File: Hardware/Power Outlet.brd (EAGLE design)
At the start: 160 x 100 mm, 36 parts, among them IC1 ATMega 328p-pu, IC2 ULN2003AD, K1 G5LE, K2 G5LE, Q1 16MHz

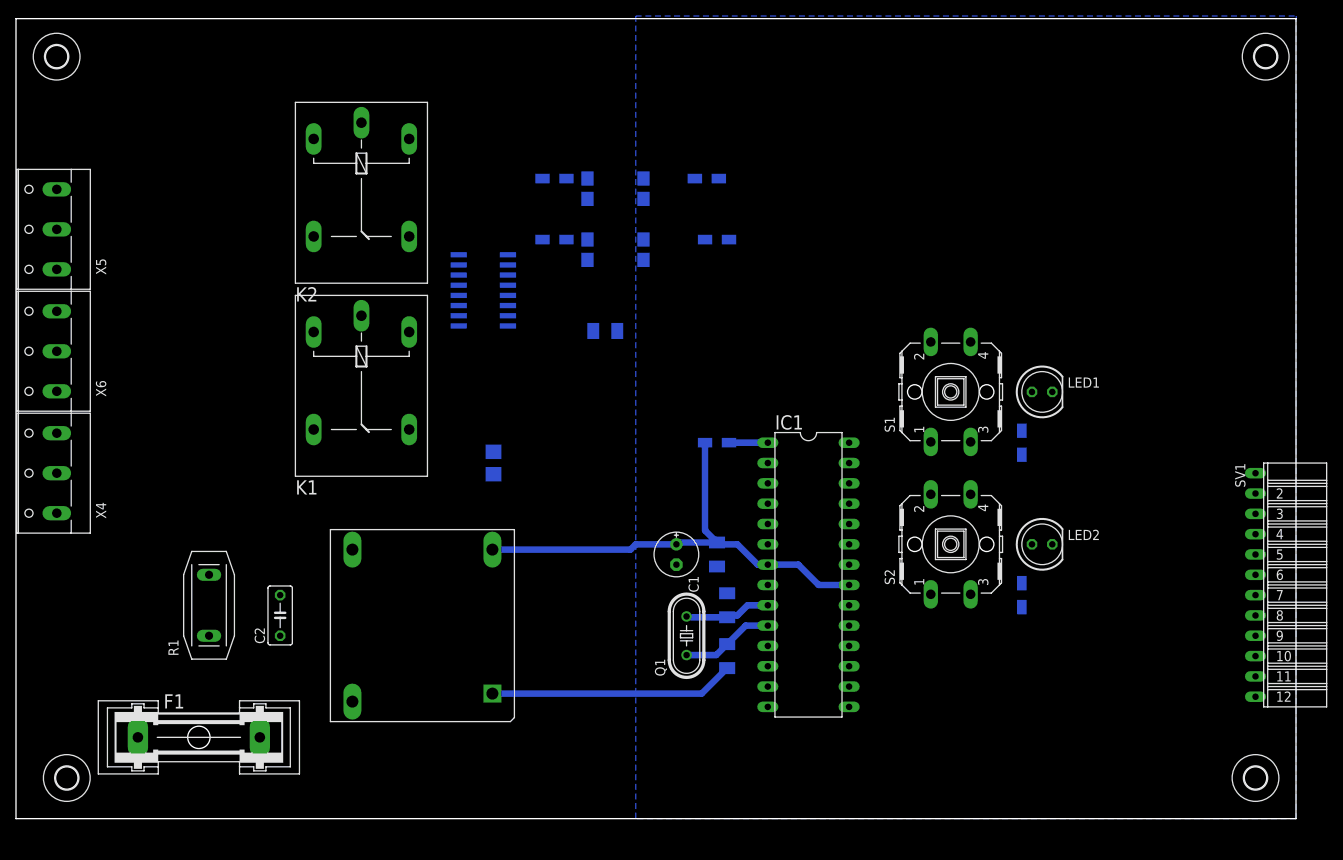
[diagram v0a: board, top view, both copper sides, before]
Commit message: Finilised Rev A. Power Outlet Board
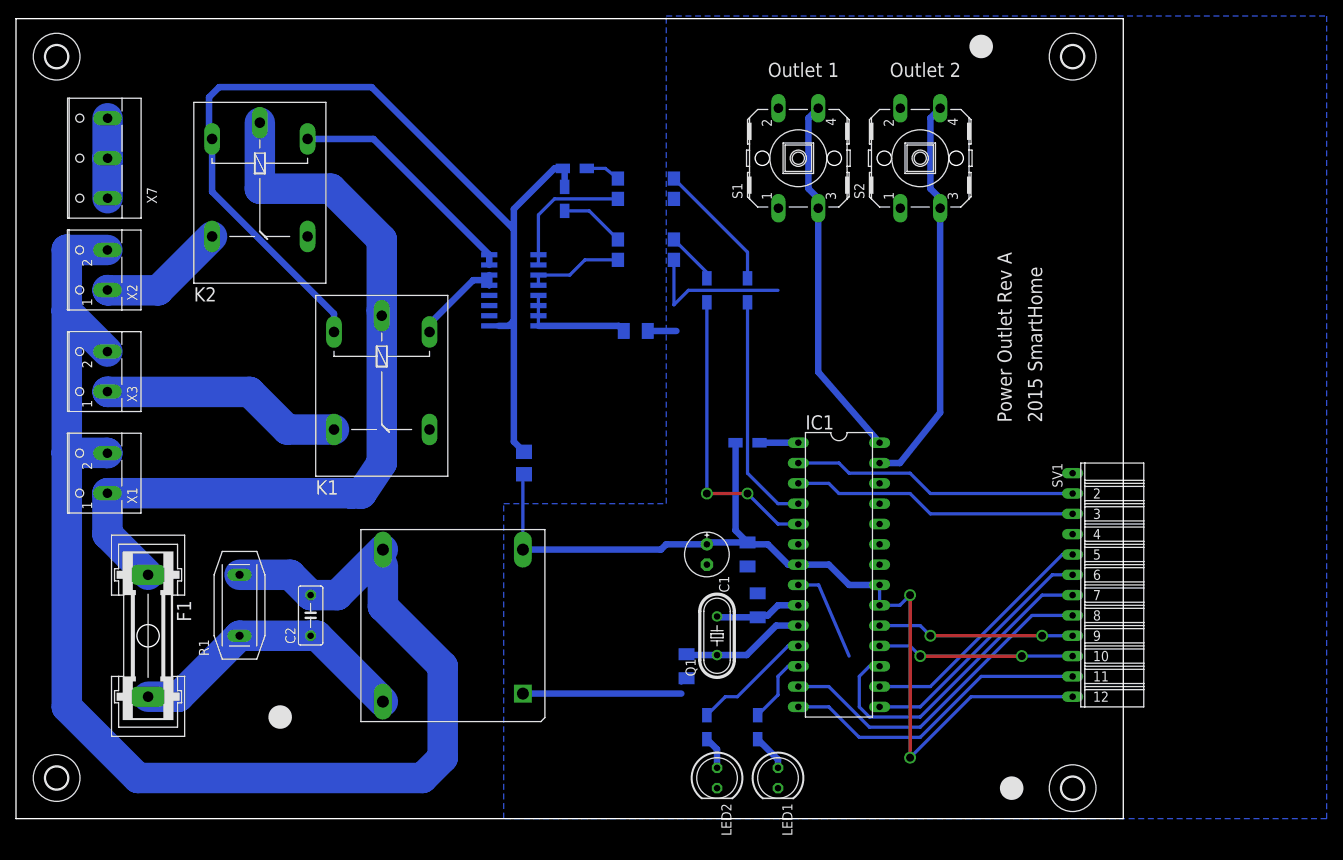
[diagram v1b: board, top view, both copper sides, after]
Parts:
- removed X4, X5, X6: (no value), con-wago-500:W237-103
- added X1: VIN, con-wago-500:W237-102
- added X2: VOUT2, con-wago-500:W237-102
- added X3: VOUT1, con-wago-500:W237-102
- added X7: EARTH, con-wago-500:W237-103
- moved LED1 58.5 mm to (95.2, 5.08), turned to 270 degrees
- moved LED2 50.0 mm to (87.6, 5.08), turned to 270 degrees
- moved R3 48.5 mm to (92.7, 11.4), turned to 90 degrees
- moved S2 48.4 mm to (113.0, 82.5)
- moved R4 42.7 mm to (86.4, 11.4), turned to 90 degrees
- moved S1 34.9 mm to (97.8, 82.5)
- moved H3 24.1 mm to (132.1, 95.2)
- moved H2 22.9 mm to (132.1, 3.81)
- moved SV1 22.9 mm to (132.1, 29.2)
- moved R5 14.9 mm to (91.4, 66.0), turned to 270 degrees
- moved F1 14.2 mm to (16.5, 22.9), turned to 270 degrees
- moved K2 12.7 mm to (30.5, 77.5)
- moved R6 6.48 mm to (86.4, 66.0), turned to 270 degrees
- moved C4 5.24 mm to (83.8, 19.1)
- moved R8 5.24 mm to (68.6, 77.5), turned to 270 degrees
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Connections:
- net GND1: now also X7.1, X7.2, X7.3; no longer X4.3, X5.3, X6.3
- net N$1: now also X1.1; no longer X4.1
- net N$11: now also X2.1; no longer X5.1
- net N$14: now also X3.1; no longer X6.1
- net N$3: now also X1.2, X2.2, X3.2; no longer X4.2, X5.2, X6.2
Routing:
- net N$3: track 0.00 -> 176.7 mm
- net VCC: track 0.00 -> 126.6 mm
- net N$1: track 0.00 -> 103.4 mm
- net +3V3: track 60.2 -> 120.4 mm, vias 0 -> 2
- net N$10: track 0.00 -> 49.7 mm
- net N$9: track 0.00 -> 45.7 mm
- net INT: track 0.00 -> 42.2 mm
- net MOSI: track 0.00 -> 40.4 mm
- net CSN2: track 0.00 -> 39.0 mm
- net OUT1_R: track 0.00 -> 36.9 mm, vias 0 -> 2
- net N$2: track 0.00 -> 35.9 mm
- net RXD: track 0.00 -> 35.9 mm
- net TXD: track 0.00 -> 35.9 mm
- net CSN: track 0.00 -> 31.0 mm
- net CE: track 0.00 -> 31.0 mm
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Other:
- board size 160 x 100 mm -> 138.4 x 100 mm
- board text added: "2015"
- board text added: "Outlet 1"
- board text added: "Outlet 2"
- board text added: "Power Outlet Rev A"
- board text added: "SmartHome"
